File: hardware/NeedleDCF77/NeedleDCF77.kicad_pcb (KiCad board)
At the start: 2 copper layers, 130 x 30 mm, 95 parts, among them J1 USB_C_Receptacle_USB2.0, J2 Battery, J3 SWD, J4 UART, J5 Hours, J6 Minutes, J7 Seconds, Q1 AO3401A, Q2 AO3400A, SW1 ShowDate, U1 LTC3558, U2 STM32L051C8Tx, U3 MAS6180_77kHz, U4 LT1617, U5 PT6312, U6 LM4871, Y2 32.768kHz

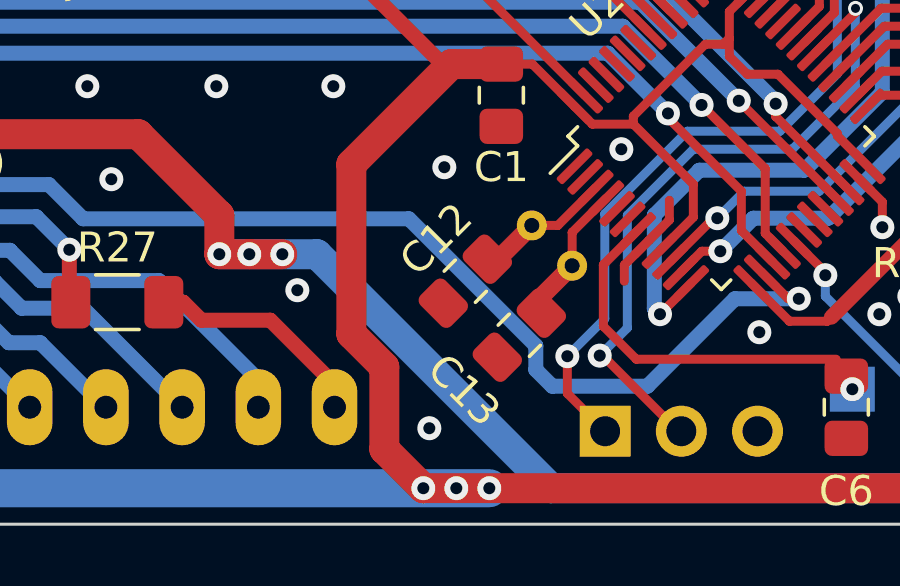
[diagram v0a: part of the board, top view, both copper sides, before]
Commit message: Update KiCad version of project
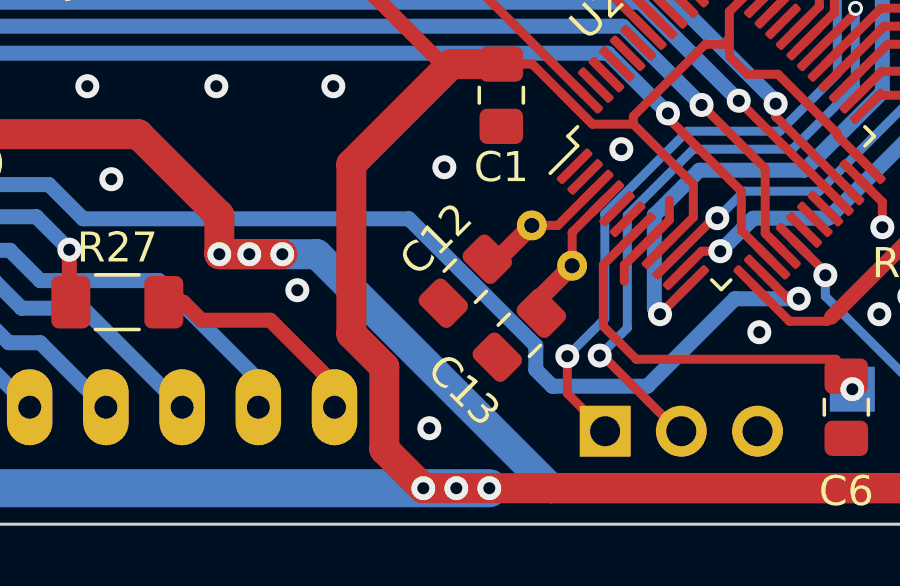
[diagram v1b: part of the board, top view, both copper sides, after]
